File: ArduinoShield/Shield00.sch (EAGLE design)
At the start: 43 parts

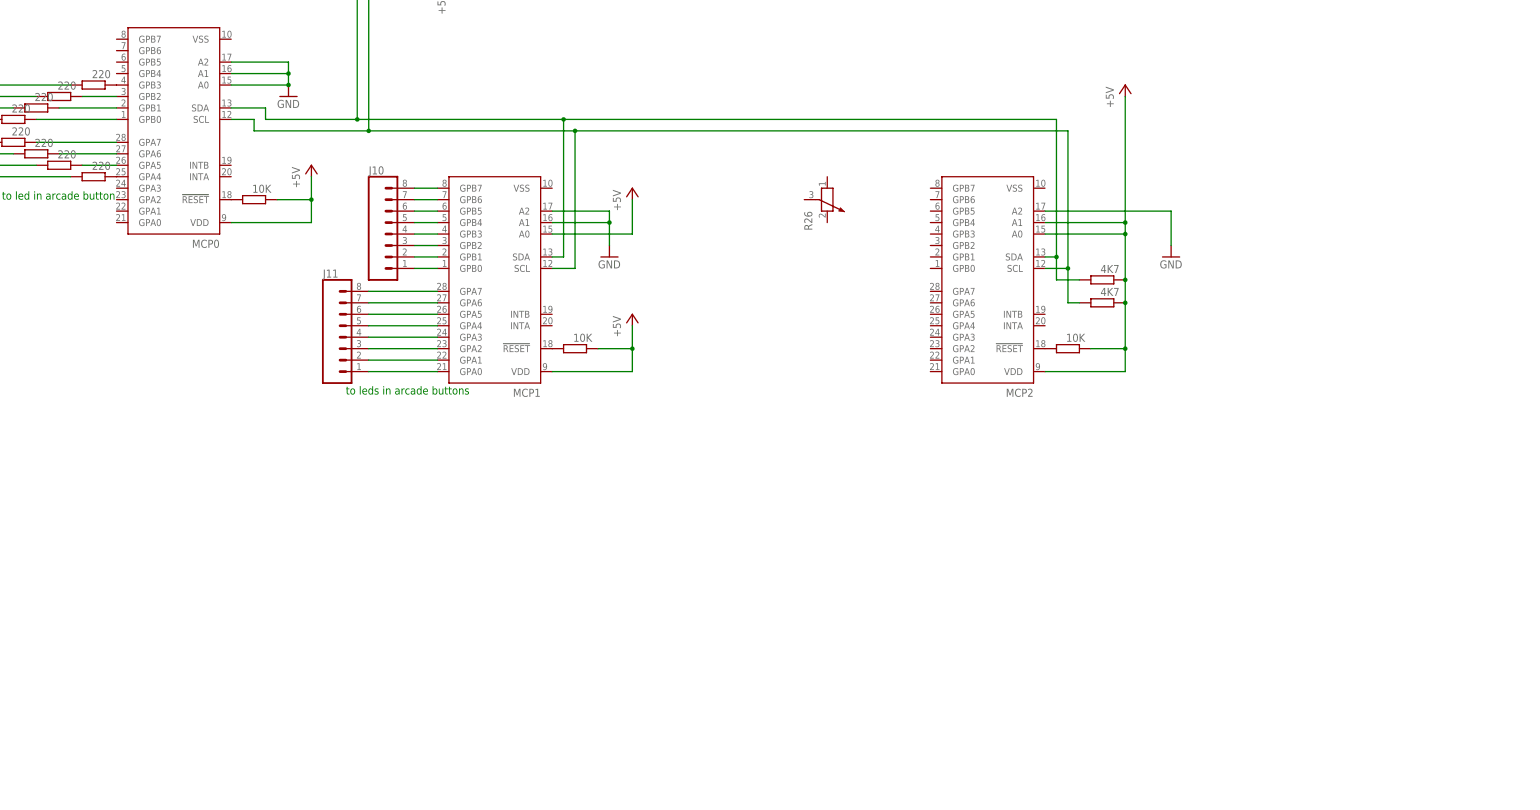
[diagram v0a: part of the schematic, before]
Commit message: end v1 schemboard
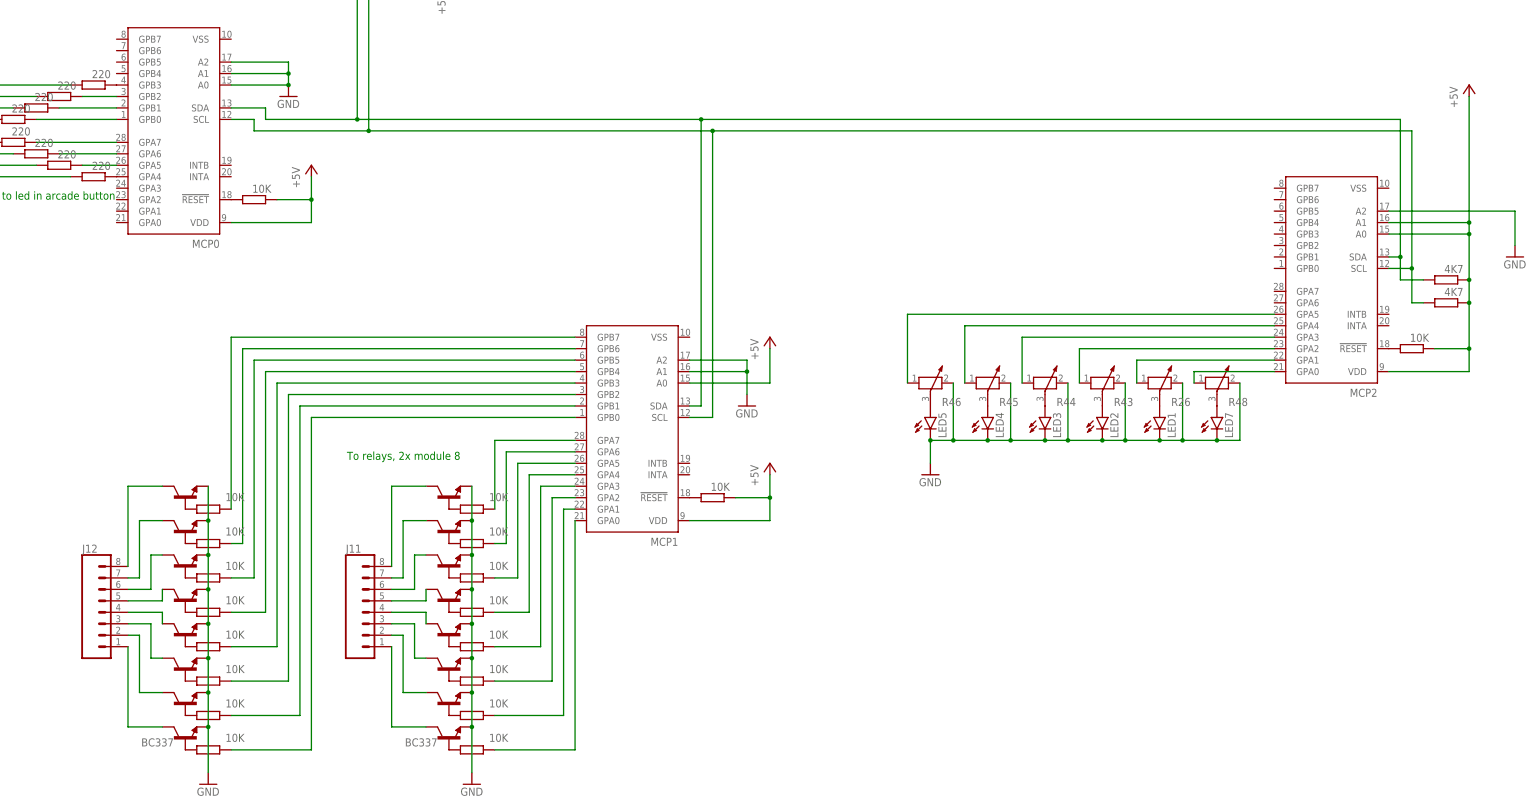
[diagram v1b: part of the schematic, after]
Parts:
- removed J10: (no value), SparkFun-Connectors:CONN_08"
- added J12: (no value), SparkFun-Connectors:CONN_08"
- added LED1, LED2, LED3, LED4, LED5, LED7: (no value), led:LED5MM
- added R27, R28, R29, R30, R31, R32, R33, R34, R35, R36, R37, R38, R39, R40, R41, R42: 10K, rcl:R-EU_R0805
- added R43, R44, R45, R46, R48: (no value), rcl:POTENTIOMETER_PT-10
- added T1, T10, T11, T12, T13, T14, T15, T16, T2, T3, T4, T5, T6, T7, T8, T9: BC337, transistor:BC337
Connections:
- new net N$53: R34.1, T8.B
- new net N$54: R36.1, T10.B
- new net N$56: R37.1, T11.B
- new net N$57: R38.1, T12.B
- new net N$58: R39.1, T13.B
- new net N$59: R40.1, T14.B
- new net N$60: R41.1, T15.B
- new net N$61: R42.1, T16.B
- new net N$62: MCP1.GPA7, R34.2
- new net N$63: MCP1.GPA6, R33.2
- new net N$64: MCP1.GPA5, R32.2
- new net N$65: MCP1.GPA4, R31.2
- new net N$66: MCP1.GPA3, R30.2
- new net N$67: MCP1.GPA2, R29.2
- new net N$68: MCP1.GPA1, R28.2
- new net N$69: MCP1.GPA0, R27.2
- new net N$70: J11.4, T4.C
- new net N$71: J11.5, T5.C
- new net N$72: J11.6, T6.C
- new net N$73: J11.7, T7.C
- new net N$74: J11.8, T8.C
- new net N$75: J11.3, T3.C
- new net N$76: J11.2, T2.C
- new net N$77: J11.1, T1.C
- new net N$78: J12.4, T12.C
- new net N$79: J12.5, T13.C
- new net N$80: J12.6, T14.C
- new net N$81: J12.7, T15.C
- new net N$82: J12.8, T16.C
- new net N$83: J12.3, T11.C
- new net N$84: J12.2, T10.C
- new net N$85: J12.1, T9.C
- new net N$86: MCP2.GPA0, R48.1
- new net N$87: LED1.A, R26.3
- new net N$88: MCP2.GPA1, R26.1
- new net N$89: LED2.A, R43.3
- new net N$90: MCP2.GPA2, R43.1
- new net N$91: LED3.A, R44.3
- new net N$92: MCP2.GPA3, R44.1
- new net N$93: LED4.A, R45.3
- new net N$94: MCP2.GPA4, R45.1
- new net N$95: LED5.A, R46.3
- new net N$96: MCP2.GPA5, R46.1
- new net N$98: LED7.A, R48.3
- net GND: now also LED1.C, LED2.C, LED3.C, LED4.C, LED5.C, LED7.C, R26.2, R43.2, R44.2, R45.2, R46.2, R48.2, T1.E, T10.E, T11.E, T12.E, T13.E, T14.E, T15.E, T16.E, T2.E, T3.E, T4.E, T5.E, T6.E, T7.E, T8.E, T9.E
- net N$37: now also R39.2; no longer J10.5
- net N$38: now also R38.2; no longer J10.4
- net N$39: now also R37.2; no longer J10.3
- net N$40: now also R36.2; no longer J10.2
- net N$41: now also R35.2; no longer J10.1
- net N$42: now also R32.1, T6.B; no longer J11.8, MCP1.GPA7
- net N$43: now also R35.1, T9.B; no longer J11.7, MCP1.GPA6
- net N$44: now also R27.1, T1.B; no longer J11.6, MCP1.GPA5
- net N$45: now also R28.1, T2.B; no longer J11.5, MCP1.GPA4
- net N$46: now also R30.1, T4.B; no longer J11.4, MCP1.GPA3
- net N$47: now also R29.1, T3.B; no longer J11.3, MCP1.GPA2
- net N$48: now also R31.1, T5.B; no longer J11.2, MCP1.GPA1
- net N$49: now also R33.1, T7.B; no longer J11.1, MCP1.GPA0
- net N$50: now also R40.2; no longer J10.6
- net N$51: now also R41.2; no longer J10.7
- net N$52: now also R42.2; no longer J10.8
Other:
- note added: "To relays, 2x module 8"
- note removed: "to leds in arcade buttons"
- moved on the sheet: J11, MCP1, MCP2, R26
